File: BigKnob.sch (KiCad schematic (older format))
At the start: 7 parts, among them J1 NSJ12HF-1, J2 NSJ12HF-1, J3 NSJ12HF-1, J4 STEREO-JACK-SWITCHED-5-Pin, J5 STEREO-JACK-SWITCHED-5-Pin

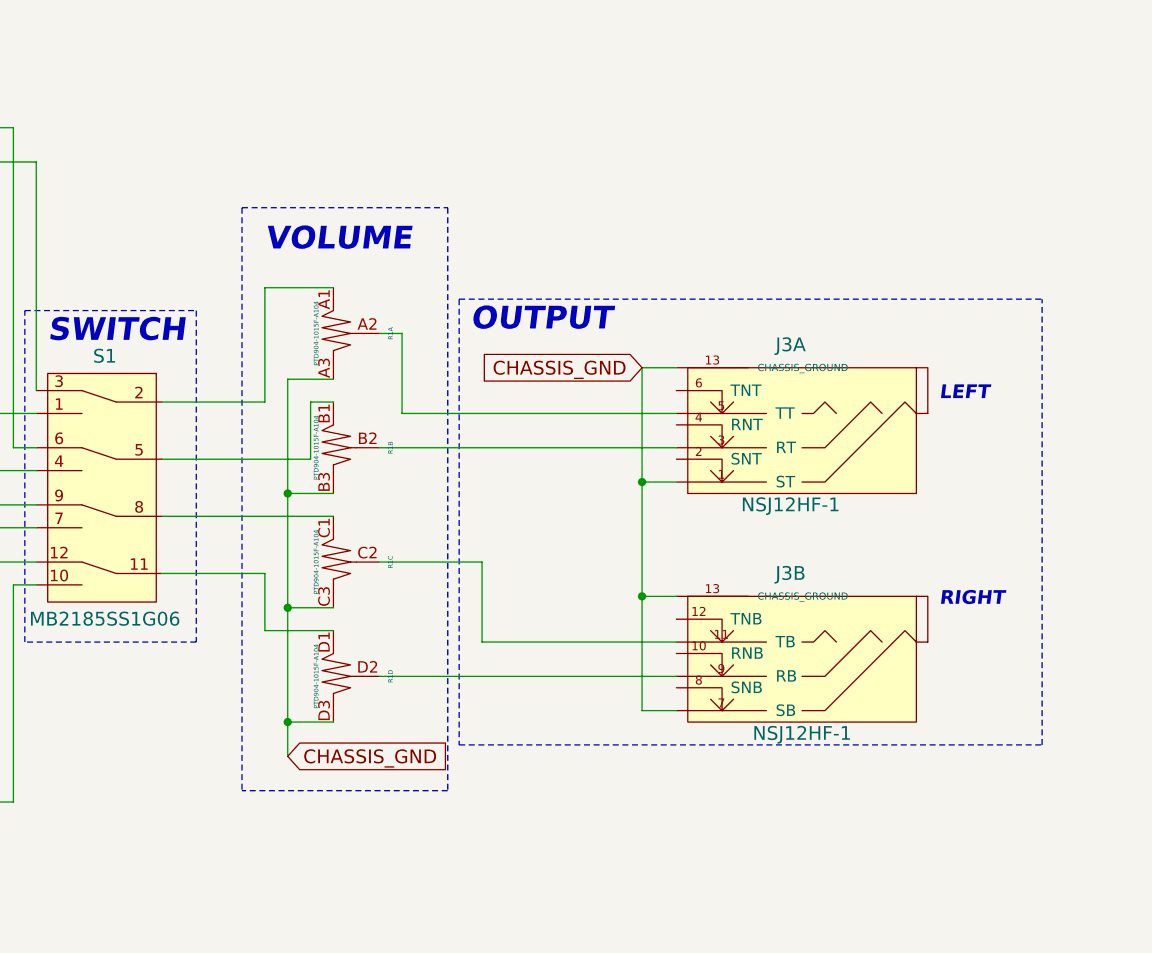
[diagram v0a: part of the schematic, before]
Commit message: :punch: v1.1
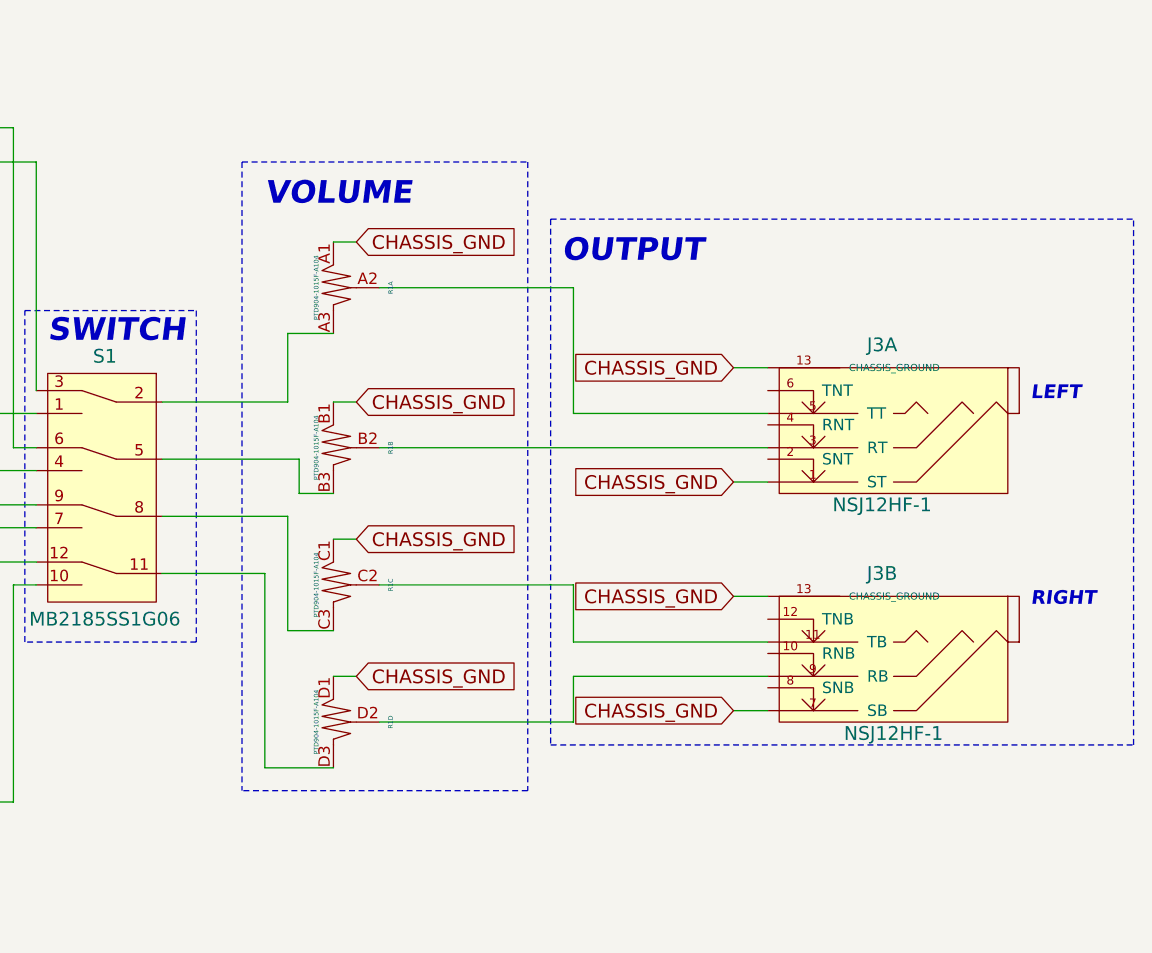
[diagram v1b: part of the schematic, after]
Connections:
- net CHASSIS_GND: now also R1.A1, R1.B1, R1.C1, R1.D1; no longer R1.A3, R1.B3, R1.C3, R1.D3
- net at S1.11: now also R1.D3; no longer R1.D1
- net at S1.2: now also R1.A3; no longer R1.A1
- net at S1.5: now also R1.B3; no longer R1.B1
- net at S1.8: now also R1.C3; no longer R1.C1
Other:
- moved on the sheet: J3A, J3B, R1A, R1C, R1D
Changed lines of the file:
@@
 L NSJ12HF-1 J3
 U 1 1 58E15C9F
-P 8350 3700
-F 0 "J3" H 8400 3300 60  0000 C CNN
-F 1 "NSJ12HF-1" H 8400 4000 60  0000 C CNN
-F 2 "stahllabs:NSJ12HF-1" H 8700 3850 60  0001 C CNN
-F 3 "http://www.neutrik.com/en/audio/plugs-and-jacks/stacking-jacks/nsj12hf-1" H 8400 3200 21  0001 C BIN
-	1    8350 3700
+P 8750 3700
+F 0 "J3" H 8800 3300 60  0000 C CNN
+F 1 "NSJ12HF-1" H 8800 4000 60  0000 C CNN
+F 2 "stahllabs:NSJ12HF-1" H 9100 3850 60  0001 C CNN
+F 3 "http://www.neutrik.com/en/audio/plugs-and-jacks/stacking-jacks/nsj12hf-1" H 8800 3200 21  0001 C BIN
+	1    8750 3700
 	-1   0    0    1
 $EndComp
@@
 L NSJ12HF-1 J3
 U 2 1 58E15D3A
-P 8350 4700
-F 0 "J3" H 8400 4300 60  0000 C CNN
-F 1 "NSJ12HF-1" H 8350 5000 60  0000 C CNN
-F 2 "stahllabs:NSJ12HF-1" H 8700 4850 60  0001 C CNN
-F 3 "http://www.neutrik.com/en/audio/plugs-and-jacks/stacking-jacks/nsj12hf-1" H 8400 4200 21  0001 C BIN
-	2    8350 4700
+P 8750 4700
+F 0 "J3" H 8800 4300 60  0000 C CNN
+F 1 "NSJ12HF-1" H 8750 5000 60  0000 C CNN
+F 2 "stahllabs:NSJ12HF-1" H 9100 4850 60  0001 C CNN
+F 3 "http://www.neutrik.com/en/audio/plugs-and-jacks/stacking-jacks/nsj12hf-1" H 8800 4200 21  0001 C BIN
+	2    8750 4700
 	-1   0    0    1
 $EndComp
 Wire Wire Line
-	6950 4250 6950 4600
-Wire Wire Line
-	6950 4600 7800 4600
-Wire Wire Line
-	6500 4750 7800 4750
+	7350 4350 7350 4600
+Wire Wire Line
+	7350 4600 8200 4600
 Wire Wire Line
 	3150 4550 4550 4550
@@
 Wire Wire Line
 	4550 4550 4550 6500
-Text Notes 8950 3550 0    60   Italic 12
+Text Notes 9350 3550 0    60   Italic 12
 LEFT
 Text Notes 1800 2650 0    60   Italic 12
@@
 RIGHT
 Wire Wire Line
-	7650 4400 7800 4400
-Wire Wire Line
-	7650 3400 7650 3900
-Wire Wire Line
-	7650 3900 7650 4400
-Wire Wire Line
-	7650 4400 7650 4900
-Wire Wire Line
-	7800 3900 7650 3900
-Connection ~ 7650 3900
-Wire Wire Line
-	7650 4900 7800 4900
-Connection ~ 7650 4400
-Text Notes 8950 4450 0    60   Italic 12
+	8050 4400 8200 4400
+Wire Wire Line
+	8200 3900 8050 3900
+Wire Wire Line
+	8050 4900 8200 4900
+Text Notes 9350 4450 0    60   Italic 12
 RIGHT
 Wire Wire Line
@@
 Connection ~ 3300 3600
 Wire Wire Line
-	7650 3400 7800 3400
-Text GLabel 7650 3400 0    60   Input ~ 0
+	8050 3400 8200 3400
+Text GLabel 8050 3400 0    60   Input ~ 0
 CHASSIS_GND
 Wire Wire Line
@@
 	3150 5300 4900 5300
 Wire Notes Line
-	6850 3100 9400 3100
-Wire Notes Line
-	6850 3100 6850 5050
-Wire Notes Line
-	6850 5050 9400 5050
-Wire Notes Line
-	9400 5050 9400 3100
-Text Notes 6900 3250 0    99   Italic 20
+	7250 2750 9800 2750
+Wire Notes Line
+	7250 2750 7250 5050
+Wire Notes Line
+	7250 5050 9800 5050
+Wire Notes Line
+	9800 5050 9800 2750
+Text Notes 7300 2950 0    99   Italic 20
 OUTPUT
 $Comp
@@
 Text Notes 1450 1300 0    99   Italic 20
 INPUT A\nmini jack
-Wire Wire Line
-	5550 4050 6300 4050
-Text GLabel 6100 5100 2    60   Input ~ 0
+Text GLabel 6400 4750 2    60   Input ~ 0
 CHASSIS_GND
 $Comp
 L PTD904-1015F-A104 R1
 U 1 1 58FEAB86
-P 6300 3250
-F 0 "R1" H 6300 3500 20  0000 C CNN
-F 1 "PTD904-1015F-A104" H 6300 3175 20  0000 C CNN
-F 2 "stahllabs:PTD904-1015F-A104" H 6300 3250 60  0001 C CNN
-F 3 "" H 6300 3250 60  0001 C CNN
-	1    6300 3250
+P 6300 3050
+F 0 "R1" H 6300 3300 20  0000 C CNN
+F 1 "PTD904-1015F-A104" H 6300 2975 20  0000 C CNN
+F 2 "stahllabs:PTD904-1015F-A104" H 6300 3050 60  0001 C CNN
+F 3 "" H 6300 3050 60  0001 C CNN
+	1    6300 3050
 	0    1    1    0
 $EndComp
@@
 L PTD904-1015F-A104 R1
 U 4 1 58FEAC80
-P 6300 4750
-F 0 "R1" H 6300 5000 20  0000 C CNN
-F 1 "PTD904-1015F-A104" H 6300 4675 20  0000 C CNN
-F 2 "stahllabs:PTD904-1015F-A104" H 6300 4750 60  0001 C CNN
-F 3 "" H 6300 4750 60  0001 C CNN
-	4    6300 4750
+P 6300 4950
+F 0 "R1" H 6300 5200 20  0000 C CNN
+F 1 "PTD904-1015F-A104" H 6300 4875 20  0000 C CNN
+F 2 "stahllabs:PTD904-1015F-A104" H 6300 4950 60  0001 C CNN
+F 3 "" H 6300 4950 60  0001 C CNN
+	4    6300 4950
 	0    1    1    0
 $EndComp
@@
 SWITCH
 Wire Notes Line
-	5900 2700 6800 2700
-Wire Notes Line
-	5900 2700 5900 5250
-Text Notes 6000 2900 0    99   Italic 20
+	5900 2500 7150 2500
+Wire Notes Line
+	5900 2500 5900 5250
+Text Notes 6000 2700 0    99   Italic 20
 VOLUME
-Wire Wire Line
-	6600 3250 6600 3600
-Wire Wire Line
-	6600 3600 7800 3600
-Wire Wire Line
-	6500 3750 7800 3750
 $Comp
 L PTD904-1015F-A104 R1
 U 3 1 58FEAC45
-P 6300 4250
-F 0 "R1" H 6300 4500 20  0000 C CNN
-F 1 "PTD904-1015F-A104" H 6300 4175 20  0000 C CNN
-F 2 "stahllabs:PTD904-1015F-A104" H 6300 4250 60  0001 C CNN
-F 3 "" H 6300 4250 60  0001 C CNN
-	3    6300 4250
+P 6300 4350
+F 0 "R1" H 6300 4600 20  0000 C CNN
+F 1 "PTD904-1015F-A104" H 6300 4275 20  0000 C CNN
+F 2 "stahllabs:PTD904-1015F-A104" H 6300 4350 60  0001 C CNN
+F 3 "" H 6300 4350 60  0001 C CNN
+	3    6300 4350
 	0    1    1    0
 $EndComp
 Wire Wire Line
-	5550 3550 6000 3550
-Wire Wire Line
-	6000 3550 6000 3050
-Wire Wire Line
-	6000 3050 6300 3050
-Wire Wire Line
-	6500 3250 6600 3250
+	6400 2850 6300 2850
+Wire Wire Line
+	6500 3050 7350 3050
 Wire Wire Line
 	5550 4300 6000 4300
 Wire Wire Line
-	6000 4300 6000 4550
-Wire Wire Line
-	6000 4550 6300 4550
-Wire Wire Line
-	5550 3800 6200 3800
-Wire Wire Line
-	6200 3800 6200 3550
-Wire Wire Line
-	6200 3550 6300 3550
-Wire Notes Line
-	6800 2700 6800 5250
-Wire Wire Line
-	7450 3750 7450 3750
-Wire Wire Line
-	6950 4250 6500 4250
-Wire Wire Line
-	6100 3450 6100 3950
-Wire Wire Line
-	6100 3950 6100 4450
-Wire Wire Line
-	6100 4450 6100 4950
-Wire Wire Line
-	6100 4950 6100 5100
-Wire Wire Line
-	6100 3450 6300 3450
-Wire Wire Line
-	6300 3950 6100 3950
-Connection ~ 6100 3950
-Wire Wire Line
-	6300 4450 6100 4450
-Connection ~ 6100 4450
-Wire Wire Line
-	6300 4950 6100 4950
-Connection ~ 6100 4950
-Wire Notes Line
-	6800 5250 5900 5250
+	6000 4300 6000 5150
+Wire Wire Line
+	6400 3550 6300 3550
+Wire Notes Line
+	7150 2500 7150 5250
+Wire Wire Line
+	7850 3750 7850 3750
+Wire Wire Line
+	7350 4350 6500 4350
+Wire Notes Line
+	7150 5250 5900 5250
+Wire Wire Line
+	6100 3800 6100 3800
+Wire Wire Line
+	5550 4050 6100 4050
+Wire Wire Line
+	6100 4050 6100 4550
+Wire Wire Line
+	6100 4550 6300 4550
+Wire Wire Line
+	6000 5150 6300 5150
+Wire Wire Line
+	6400 4150 6300 4150
+Wire Wire Line
+	6300 4750 6400 4750
+Wire Wire Line
+	6500 3750 8200 3750
+Wire Wire Line
+	6100 3550 5550 3550
+Wire Wire Line
+	6500 4950 7350 4950
+Wire Wire Line
+	7350 4950 7350 4750
+Wire Wire Line
+	7350 4750 8200 4750
+Wire Wire Line
+	7350 3600 8200 3600
+Wire Wire Line
+	7350 3050 7350 3600
+Wire Wire Line
+	5550 3800 6150 3800
+Wire Wire Line
+	6150 3800 6150 3950
+Wire Wire Line
+	6150 3950 6300 3950
+Wire Wire Line
+	6100 3550 6100 3250
+Wire Wire Line
+	6100 3250 6300 3250
+Text GLabel 8050 3900 0    60   Input ~ 0
+CHASSIS_GND
+Text GLabel 8050 4400 0    60   Input ~ 0
+CHASSIS_GND
+Text GLabel 8050 4900 0    60   Input ~ 0
+CHASSIS_GND
+Text GLabel 6400 4150 2    60   Input ~ 0
+CHASSIS_GND
+Text GLabel 6400 3550 2    60   Input ~ 0
+CHASSIS_GND
+Text GLabel 6400 2850 2    60   Input ~ 0
+CHASSIS_GND
 $EndSCHEMATC

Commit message: v1.1
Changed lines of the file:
@@
 $EndComp
 Wire Wire Line
-	3150 2700 3300 2700
+	3150 2700 3500 2700
 Wire Wire Line
-	3300 2700 3500 2700
+	3150 3600 3500 3600
 Wire Wire Line
-	3150 3600 3300 3600
-Wire Wire Line
-	3300 3600 3500 3600
-Wire Wire Line
-	3150 4750 3300 4750
-Wire Wire Line
-	3300 4750 3500 4750
+	3150 4750 3500 4750
 Text GLabel 3500 2700 2    60   Input ~ 0
 CHASSIS_GND
@@
 CHASSIS_GND
 Wire Wire Line
-	3150 5650 3300 5650
-Wire Wire Line
-	3300 5650 3500 5650
+	3150 5650 3500 5650
 Text GLabel 3500 5650 2    60   Input ~ 0
 CHASSIS_GND
@@
 	3150 4550 4550 4550
 Wire Wire Line
-	4550 3600 4550 4550
-Wire Wire Line
-	4550 4550 4550 6500
+	4550 3600 4550 6500
 Text Notes 9350 3550 0    60   Italic 12
 LEFT
@@
 RIGHT
 Wire Wire Line
-	3150 2500 4450 2500
-Wire Wire Line
-	4450 2500 5000 2500
+	3150 2500 5000 2500
 Wire Wire Line
 	5000 2500 5000 3500
@@
 CHASSIS_GND
 Wire Wire Line
-	3150 3400 4550 3400
-Wire Wire Line
-	4550 3400 4800 3400
+	3150 3400 4800 3400
 Wire Wire Line
 	4800 3400 4800 4000
@@
 	4800 4000 5000 4000
 Wire Wire Line
-	3150 5450 4450 5450
-Wire Wire Line
-	4450 5450 4800 5450
+	3150 5450 4800 5450
 Wire Wire Line
 	4800 5450 4800 4100
